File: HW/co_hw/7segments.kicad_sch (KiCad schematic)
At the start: 44 parts, among them U2 74HC595, U3 74HC595, U4 74HC595, U5 74HC595

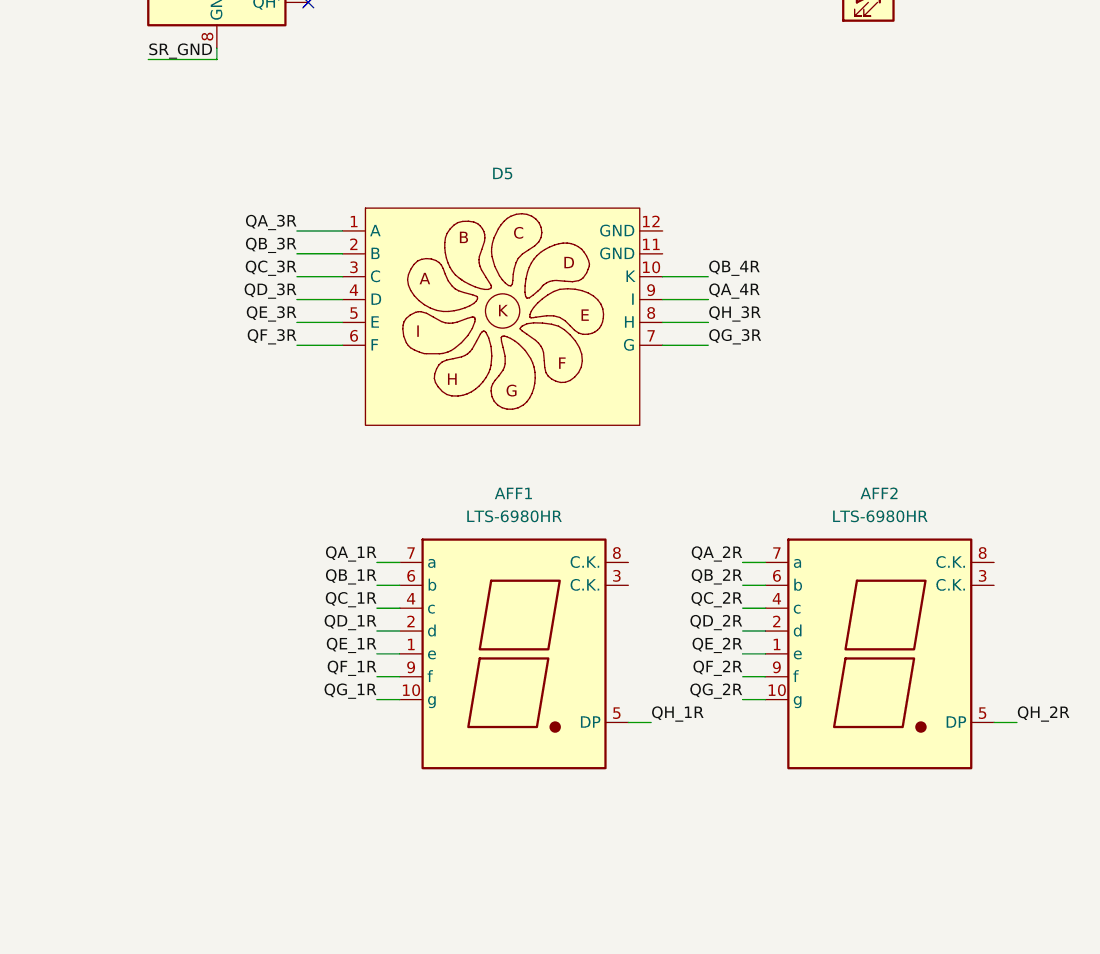
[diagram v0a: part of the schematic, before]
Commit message: HW update.
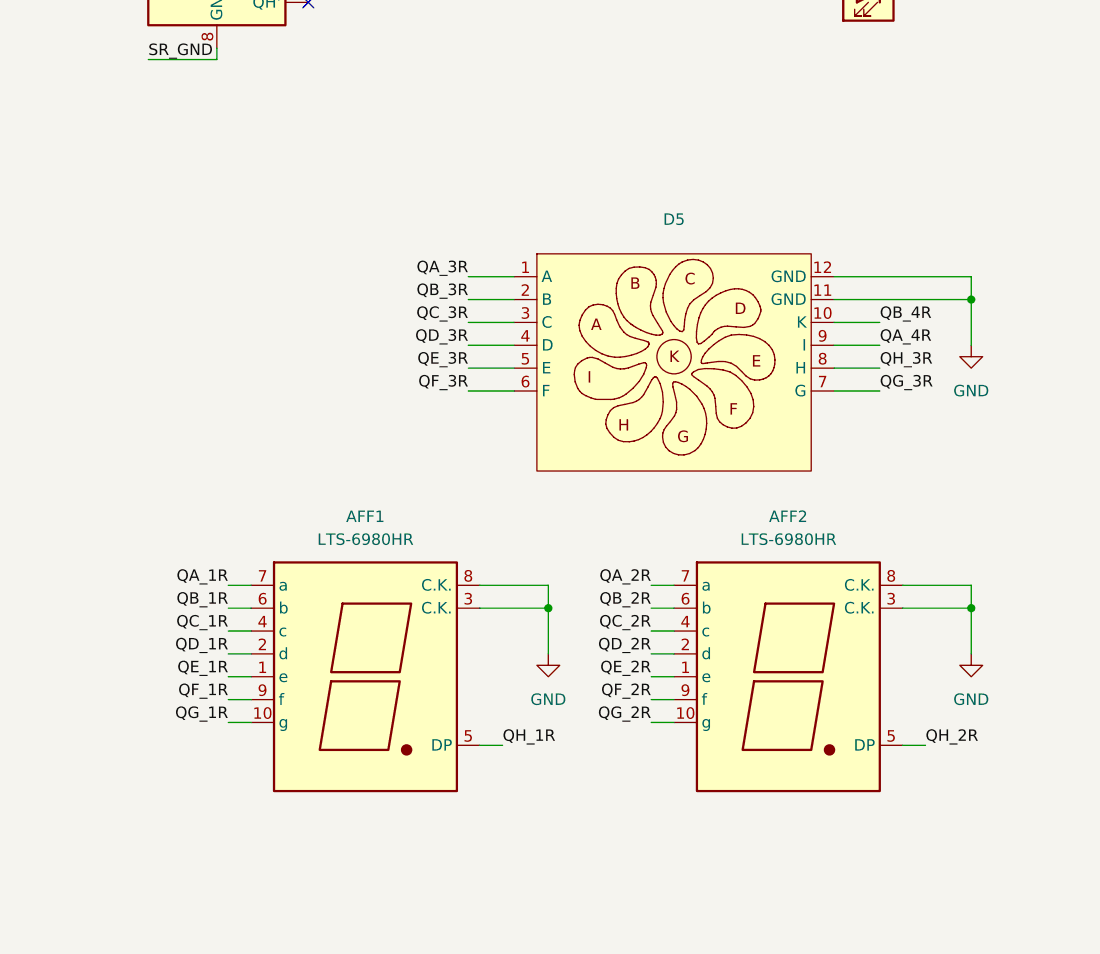
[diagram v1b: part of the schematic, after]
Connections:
- net GND: now also AFF1.3 (C.K.), AFF1.8 (C.K.), AFF2.3 (C.K.), AFF2.8 (C.K.), D5.11 (GND), D5.12 (GND)
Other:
- moved on the sheet: AFF1, AFF2, D5
